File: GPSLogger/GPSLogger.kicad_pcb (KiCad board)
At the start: 4 copper layers, 34 x 59 mm, 73 parts, among them J2 Conn_ARM_JTAG_SWD_10, J3 Micro_SD_Card, J4 USB_B_Micro, J5 BTN1, J7 Batt_Connector, Q1 Q_NMOS_GSD, SW1 Switch_SW_SPDT, U1 CAM_M8Q, U2 nRF52832-QFxx, U3 BME280, U4 BQ21040, U5 MAX17048, U6 LM3671, U7 24pin_flex_waveshare, Y1 32MHz, Y2 32.768kHz

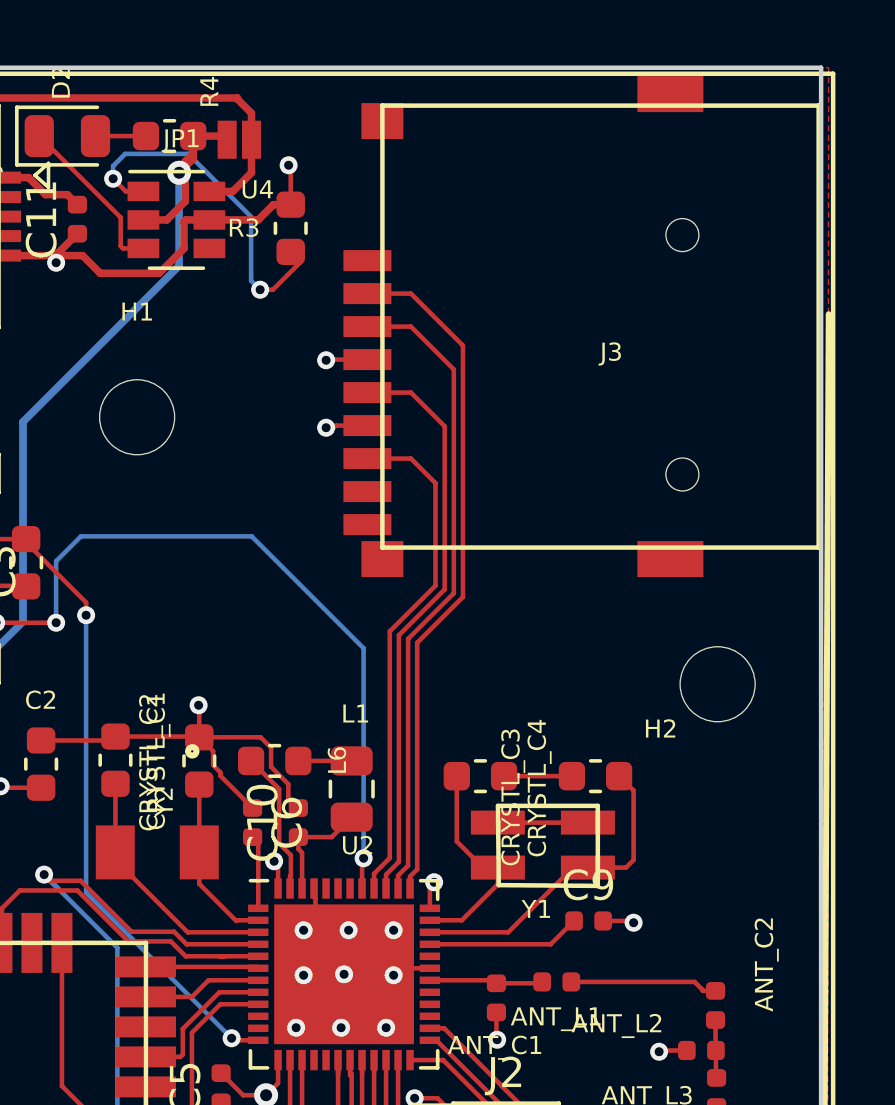
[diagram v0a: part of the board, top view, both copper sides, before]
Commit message: commit before more
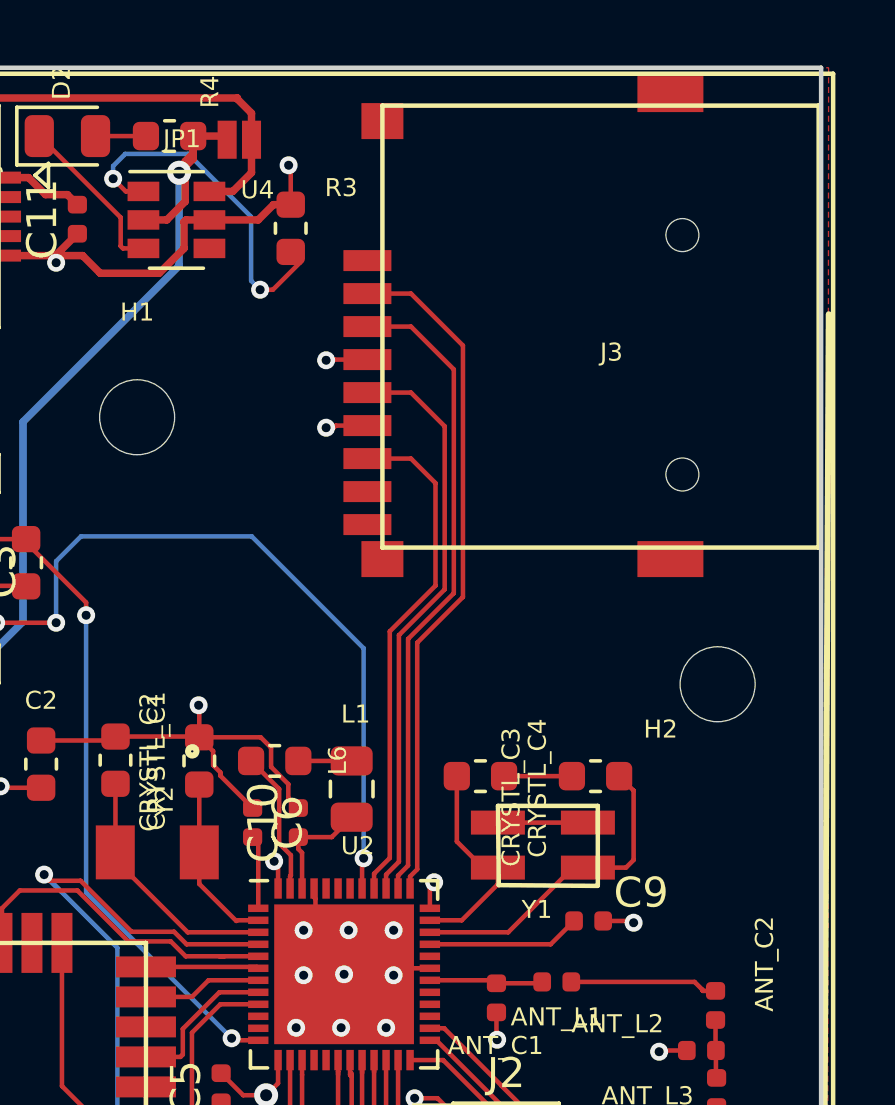
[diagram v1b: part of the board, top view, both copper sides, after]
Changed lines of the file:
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@@
   (layers
     (0 F.Cu signal)
-    (1 In1.Cu signal)
-    (2 In2.Cu signal)
-    (31 B.Cu signal)
+    (1 In1.Cu signal hide)
+    (2 In2.Cu signal hide)
+    (31 B.Cu signal hide)
     (32 B.Adhes user)
     (33 F.Adhes user)
@@
     (solder_mask_min_width 0.25)
     (aux_axis_origin 0 0)
-    (visible_elements 7FFFFEFF)
+    (visible_elements 7FFEFEFF)
     (pcbplotparams
       (layerselection 0x010fc_ffffffff)
@@
     (tags resistor)
     (attr smd)
-    (fp_text reference R3 (at 0 1.5621 180) (layer F.SilkS)
+    (fp_text reference R3 (at -1.3515 -1.68 180) (layer F.SilkS)
       (effects (font (size 0.6 0.6) (thickness 0.09)))
     )
@@
     (tags capacitor)
     (attr smd)
-    (fp_text reference C9 (at 0 -1.17) (layer F.SilkS)
+    (fp_text reference C9 (at 1.751 -0.94) (layer F.SilkS)
       (effects (font (size 1 1) (thickness 0.15)))
     )
